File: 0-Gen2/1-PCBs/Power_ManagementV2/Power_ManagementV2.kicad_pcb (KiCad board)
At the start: 2 copper layers, 70 x 94 mm, 59 parts, among them J1 Conn_01x02_Pin, J10 Conn_01x02_Pin, J2 Conn_01x02_Pin, J3 1986660-2, J4 1986660-2, J5 Conn_01x02_Pin, J6 Conn_01x02_Pin, J7 Conn_01x02_Pin, J8 Conn_01x04_Pin, J9 Conn_01x03_Pin, K2 G5V-1 DC3, Q1 MCTL160N15Y-TP, Q2 MCTL160N15Y-TP, Q3 MCTL160N15Y-TP, U1 ACS758ECB-200U-PFF-T, U2 LM393DT, U3 SN74LVC1G373DCKR, U4 74LVC1G08, U5 74LVC1G08, U6 LTC1255CS8-PBF

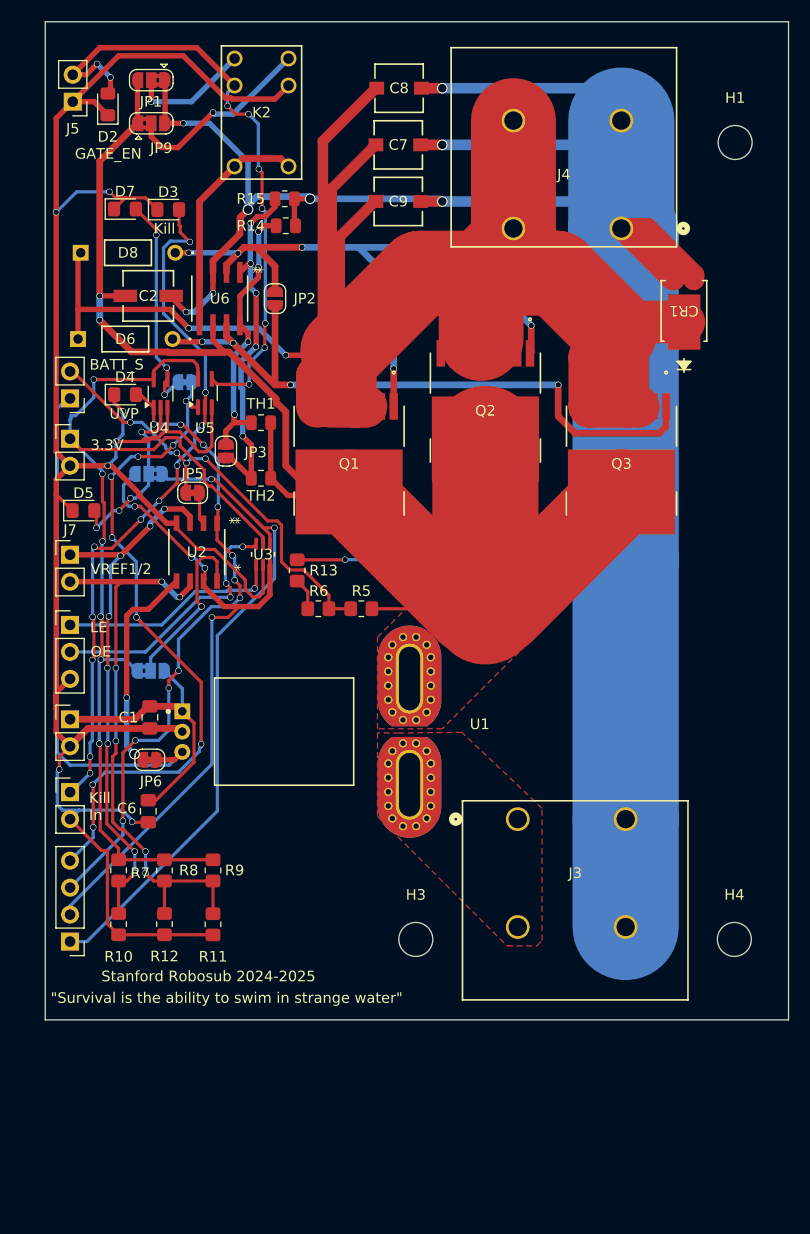
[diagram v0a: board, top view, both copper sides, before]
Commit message: almost ready to fab
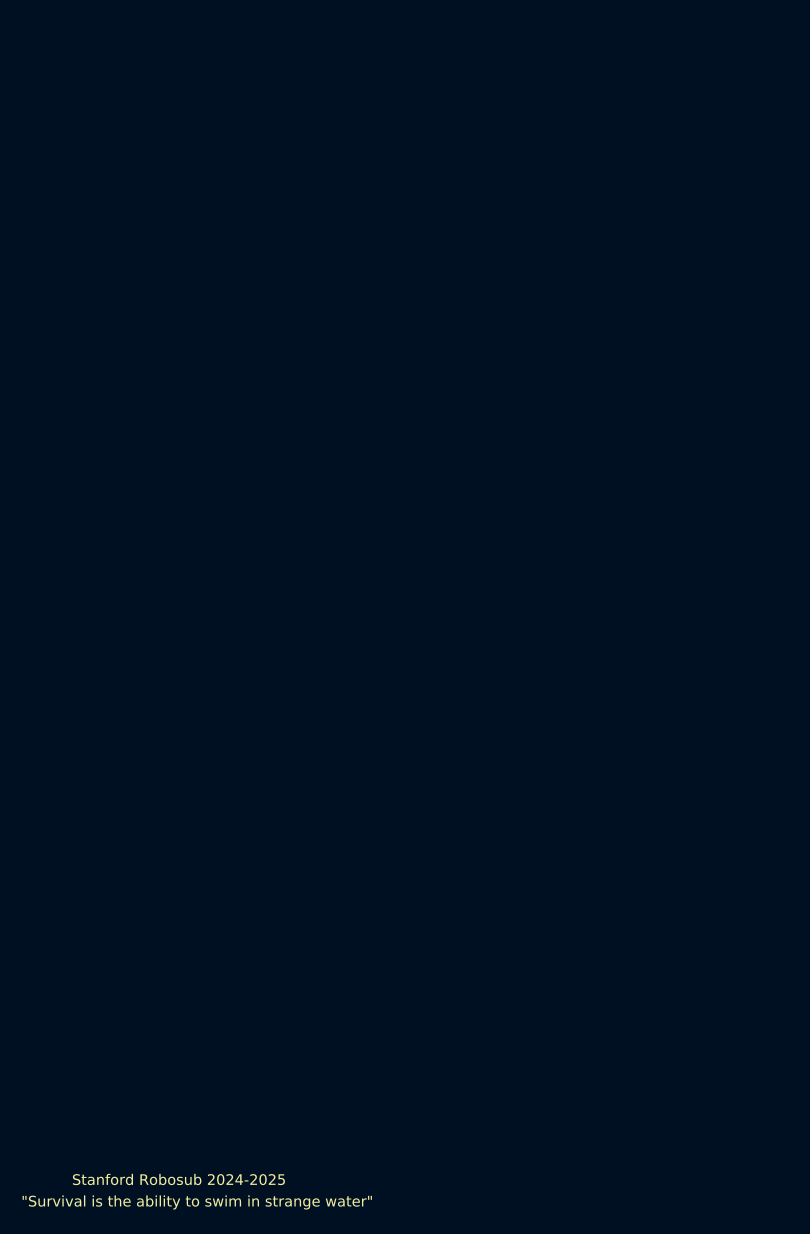
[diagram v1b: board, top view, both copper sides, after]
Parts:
- removed C1: 0.1u, Capacitor_SMD:C_0805_2012Metric_Pad1.18x1.45mm_HandSolder
- removed C2: 10uF, Imported_Footprints:CAP_EEE-1CA100SR_PAN
- removed C6: 10uF, Capacitor_SMD:C_0805_2012Metric_Pad1.18x1.45mm_HandSolder
- removed C7, C8, C9: 1u, Imported_Footprints:U2-D_NCH
- removed CR1: SBRT15U50SP5-13, Imported_Footprints:POWERDI5_DIO
- removed D2, D3, D4, D5, D7: LED, LED_SMD:LED_0805_2012Metric_Pad1.15x1.40mm_HandSolder
- removed D6, D8: D_Zener, Imported_Footprints:1N5242B
- removed H1, H3, H4: MountingHole, MountingHole:MountingHole_3.2mm_M3
- removed J1, J10, J2, J5, J6, J7: Conn_01x02_Pin, Connector_PinHeader_2.54mm:PinHeader_1x02_P2.54mm_Vertical
- removed J3, J4: 1986660-2, Imported_Footprints:CONN2_1986660-2_TEC
- removed J8: Conn_01x04_Pin, Connector_PinHeader_2.54mm:PinHeader_1x04_P2.54mm_Vertical
- removed J9: Conn_01x03_Pin, Connector_PinHeader_2.54mm:PinHeader_1x03_P2.54mm_Vertical
- removed JP1, JP4, JP7, JP9: SolderJumper_3_Bridged12, Jumper:SolderJumper-3_P1.3mm_Bridged2Bar12_RoundedPad1.0x1.5mm
- removed JP2, JP3: SolderJumper_2_Open, Jumper:SolderJumper-2_P1.3mm_Open_RoundedPad1.0x1.5mm
- removed JP5, JP6, JP8: SolderJumper_2_Bridged, Jumper:SolderJumper-2_P1.3mm_Bridged_RoundedPad1.0x1.5mm
- removed K2: G5V-1 DC3, Imported_Footprints:RELAY_G5V-1_OMR
- removed Q1, Q2, Q3: MCTL160N15Y-TP, Imported_Footprints:TOLL-8L_MCC
- removed R10: 200k, Resistor_SMD:R_0805_2012Metric_Pad1.20x1.40mm_HandSolder
- removed R11, R12, R8, R9: ~, Resistor_SMD:R_0805_2012Metric_Pad1.20x1.40mm_HandSolder
- removed R13: 500k, Resistor_SMD:R_0805_2012Metric_Pad1.20x1.40mm_HandSolder
- removed R14, R15: 100k, Resistor_SMD:R_0805_2012Metric
- removed R5, R6: 100k, Resistor_SMD:R_0805_2012Metric_Pad1.20x1.40mm_HandSolder
- removed R7: 150k, Resistor_SMD:R_0805_2012Metric_Pad1.20x1.40mm_HandSolder
- removed TH1, TH2: Thermistor_US, Resistor_SMD:R_0805_2012Metric
- removed U1: ACS758ECB-200U-PFF-T, Imported_Footprints:Allegro_MicroSystems,_LLC-CB-5-PFF-0-0-MFG
- removed U2: LM393DT, Imported_Footprints:LM393DT
- removed U3: SN74LVC1G373DCKR, Imported_Footprints:SN74LVC
- removed U4, U5: 74LVC1G08, Package_TO_SOT_SMD:SOT-353_SC-70-5_Handsoldering
- removed U6: LTC1255CS8-PBF, Imported_Footprints:LTC1255
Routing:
- net /Battery_input/-Batt: track 238.5 -> 0.00 mm, vias 9 -> 0
- net GND: track 214.0 -> 0.00 mm, vias 7 -> 0
- net /FETs/V_THRUST: track 203.8 -> 0.00 mm, vias 2 -> 0
- net /FETs/+Batt: track 133.8 -> 0.00 mm, vias 2 -> 0
- net +3.3V: track 98.5 -> 0.00 mm, vias 6 -> 0
- net /FET_control_logic/Kill_Switch: track 65.7 -> 0.00 mm, vias 11 -> 0
- net Net-(J8-Pin_4): track 64.1 -> 0.00 mm, vias 9 -> 0
- net /FET_control_logic/OCP_LATCH: track 63.2 -> 0.00 mm, vias 2 -> 0
- net /FETs/GATE2_DRIVE: track 63.1 -> 0.00 mm, vias 4 -> 0
- net /FETs/GATE1_DRIVE: track 63.0 -> 0.00 mm, vias 5 -> 0
- net /FET_control_logic/OCP_COMP: track 61.4 -> 0.00 mm, vias 4 -> 0
- net /FET_control_logic/UVP_COMP: track 61.4 -> 0.00 mm, vias 11 -> 0
- net /FET_control_logic/3.3V_GATE_EN: track 58.5 -> 0.00 mm, vias 9 -> 0
- net VREF2: track 54.9 -> 0.00 mm, vias 6 -> 0
- net VREF1: track 50.7 -> 0.00 mm, vias 8 -> 0
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- removed copper zone on F.Cu, net /Battery_input/+BATT_HALL
- removed copper zone on F.Cu, net /FETs/+Batt
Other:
- board outline removed
- board text removed: "3.3V"
- board text removed: "BATT_S"
- board text removed: "GATE_EN"
- board text removed: "Kill"
- board text removed: "Kill In"
- board text removed: "LE"
- board text removed: "OE"
- board text removed: "UVP"
- board text removed: "VREF1/2"
